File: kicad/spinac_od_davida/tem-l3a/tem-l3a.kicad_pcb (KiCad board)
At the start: 2 copper layers, 14 parts, among them J1 Conn_01x02_Male, SW1 SW_Push, SW2 SW_Push, U1 LM555xM

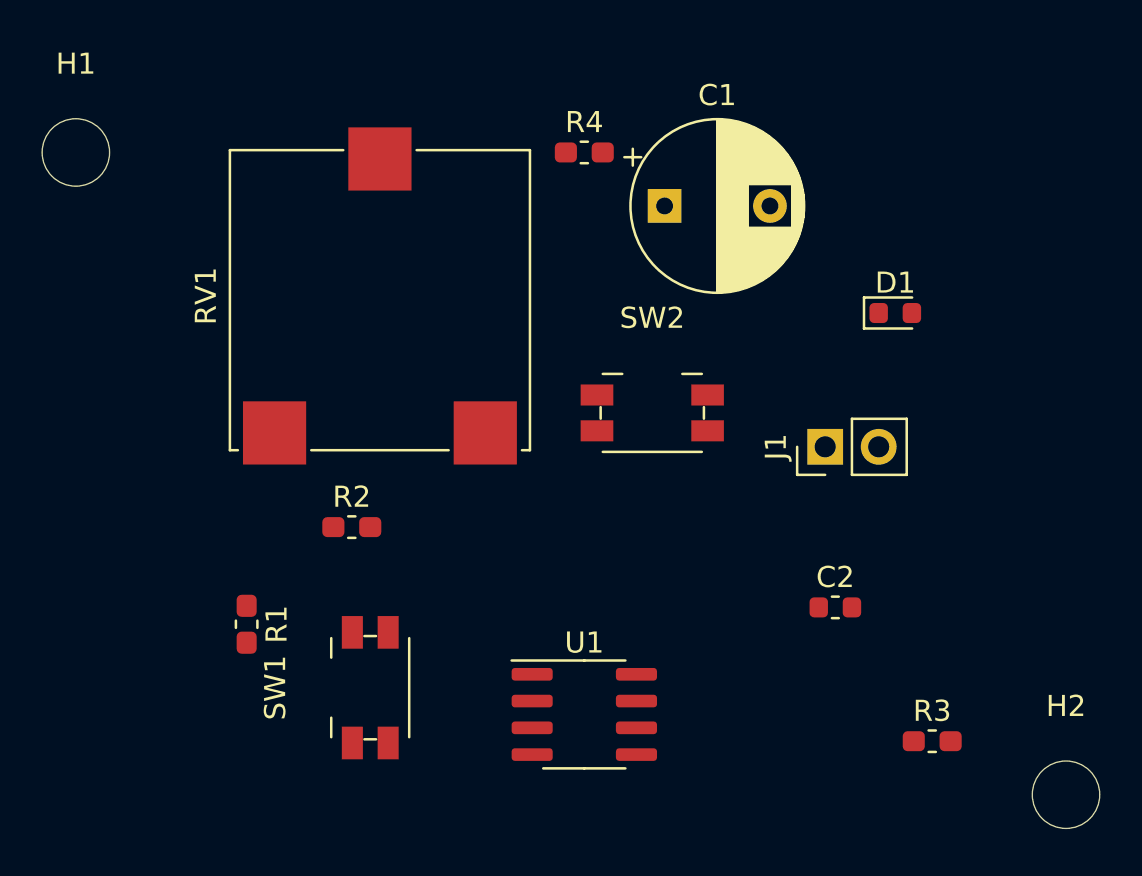
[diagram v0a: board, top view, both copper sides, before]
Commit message: 1.prosinec
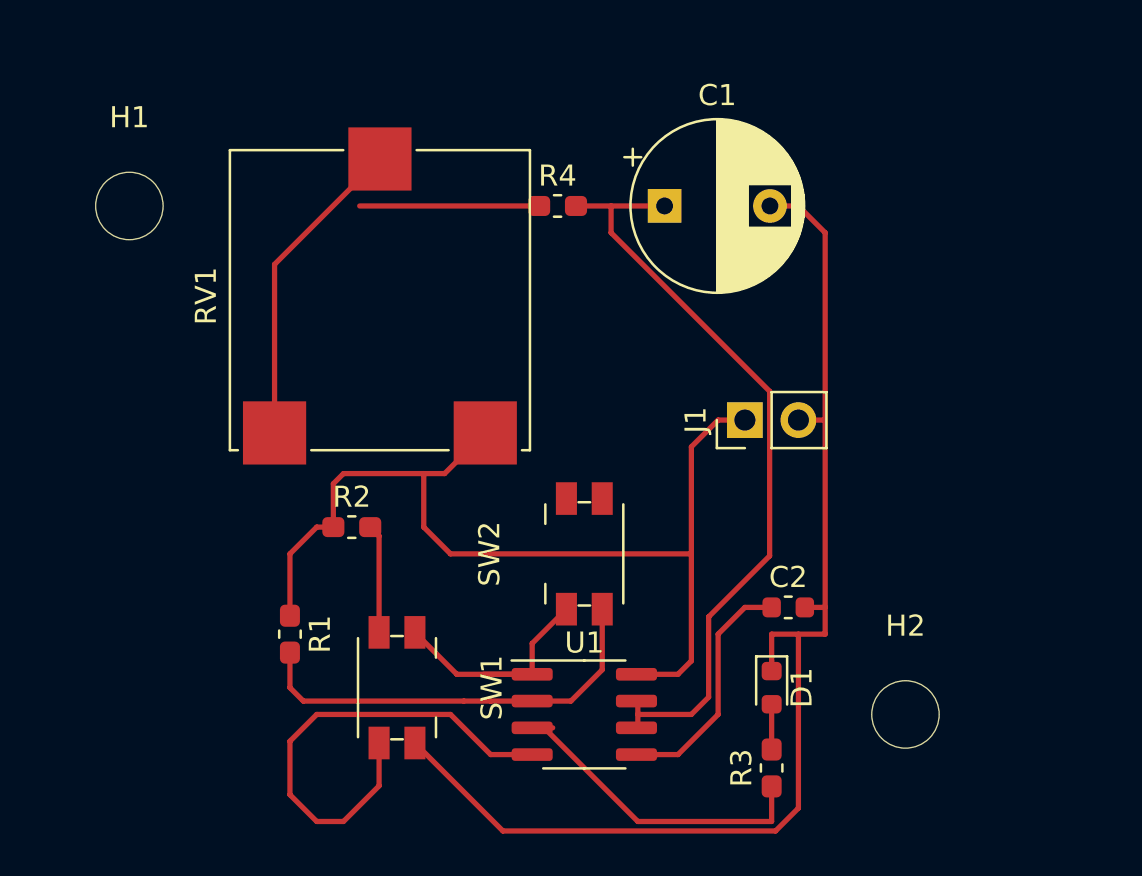
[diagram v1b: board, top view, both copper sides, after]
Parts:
- moved D1 18.7 mm to (165.1, 116.8), turned to 270 degrees
- moved H2 8.52 mm to (171.4, 118.1)
- moved R3 7.73 mm to (165.1, 120.7), turned to 90 degrees
- moved SW2 7.43 mm to (156.2, 110.5), turned to 90 degrees
- moved J1 4.02 mm to (163.8, 104.1)
- moved H1 3.59 mm to (134.6, 94.0)
- moved R4 2.84 mm to (154.9, 94.0)
- moved C2 2.24 mm to (165.9, 113.0)
- moved R1 2.11 mm to (142.2, 114.3)
- moved SW1 1.27 mm to (147.3, 116.8), turned to 270 degrees
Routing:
- net Net-(C1-Pad2): track 0.00 -> 69.8 mm
- net Net-(J1-Pad1): track 0.00 -> 47.6 mm
- net Net-(C1-Pad1): track 0.00 -> 37.2 mm
- net Net-(R2-Pad2): track 0.00 -> 28.0 mm
- net Net-(R4-Pad1): track 0.00 -> 24.0 mm
- net Net-(R1-Pad2): track 0.00 -> 20.2 mm
- net Net-(R3-Pad1): track 0.00 -> 15.8 mm
- net Net-(C2-Pad1): track 0.00 -> 12.5 mm
- net Net-(D1-Pad2): track 0.00 -> 2.15 mm

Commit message: lul
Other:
- net class Default removed
